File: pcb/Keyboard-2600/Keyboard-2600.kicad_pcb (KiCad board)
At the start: 2 copper layers, 80 x 59.7 mm, 29 parts, among them J1 USB_A, J2 Left Forward Port, J3 Right Forward Port, J4 2600 Joystick Connector, J5 Mini-DIN-6, J6 Expansion Port, SW1 Config Switch-Box, SW2 Reset, U1 ATmega328P-A, U2 74HC4066D_653, U3 74HC4066D_653, Y2 16Mhz

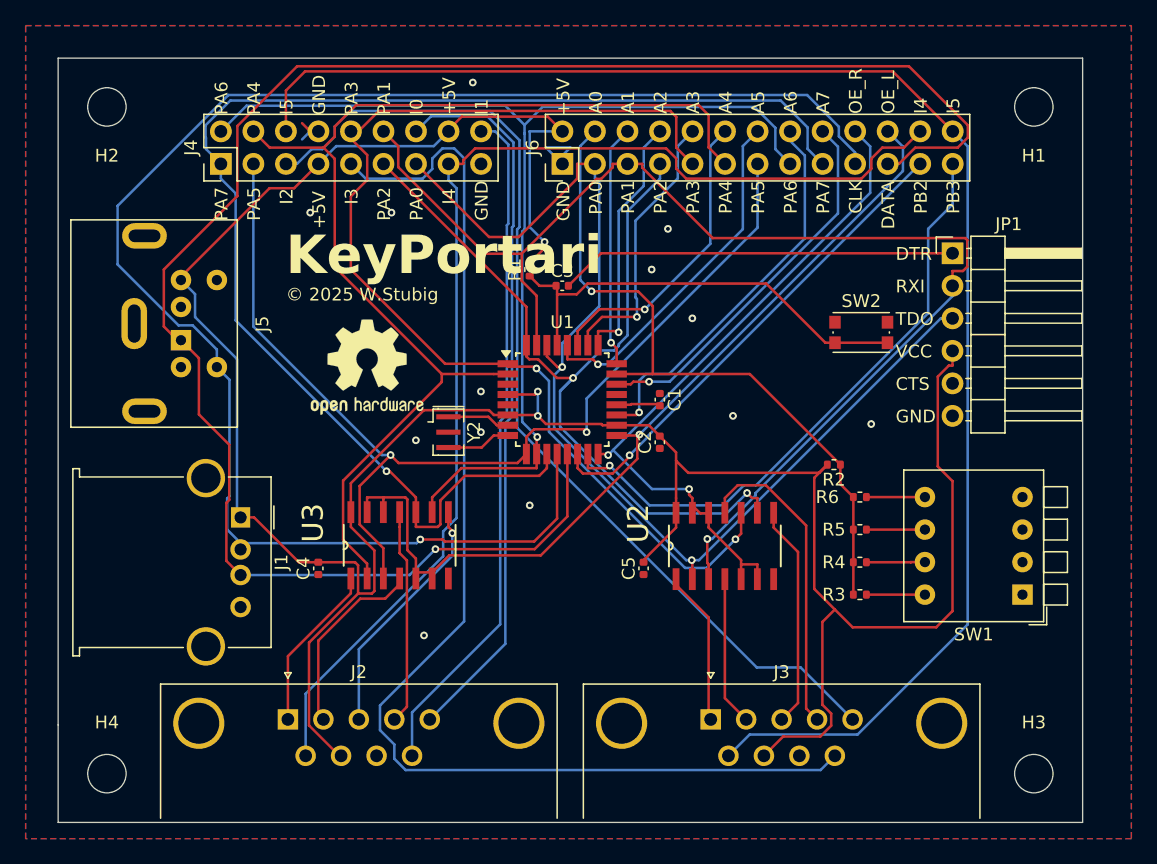
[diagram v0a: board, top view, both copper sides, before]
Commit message: Test board WIP state.
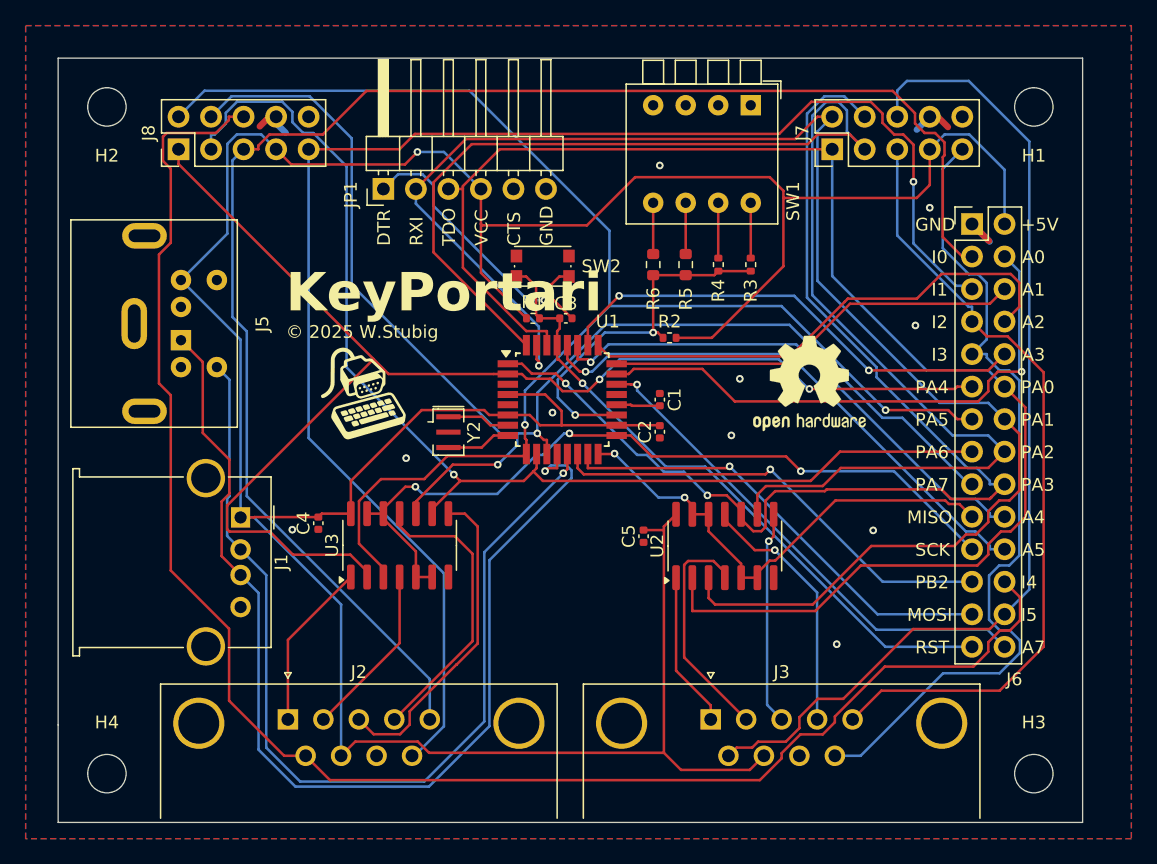
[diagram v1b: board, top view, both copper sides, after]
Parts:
- removed J4: 2600 Joystick Connector, Connector_PinHeader_2.54mm:PinHeader_2x09_P2.54mm_Vertical
- added G***: LOGO, KeyPortari:Logo KeyPortari, F.Cu at (77.5, 90.6)
- added J7: Joystick right, Connector_PinHeader_2.54mm:PinHeader_2x05_P2.54mm_Vertical, F.Cu at (113.8, 70.6)
- added J8: Joystick left, Connector_PinHeader_2.54mm:PinHeader_2x05_P2.54mm_Vertical, F.Cu at (62.7, 70.6)
- J5: footprint 2600-Keyboard:Connector_Mini-DIN_Female_6Pin_2rows -> KeyPortari:Connector_Mini-DIN_Female_6Pin_2rows
- J6: footprint Connector_PinHeader_2.54mm:PinHeader_2x13_P2.54mm_Vertical -> KeyPortari:PinHeader_2x14_P2.54mm_Vertical_KeyPortari_Expansion-Port
- R5, R6: footprint Resistor_SMD:R_0402_1005Metric -> Resistor_SMD:R_0603_1608Metric
- U2, U3: footprint 74HC4066D_653f:SOIC127P600X175-14N -> Package_SO:SOIC-14_3.9x8.7mm_P1.27mm
- moved JP1 44.7 mm to (78.7, 73.7), turned to 90 degrees
- moved SW1 43.7 mm to (107.4, 67.2), turned to -90 degrees
- moved REF** 34.6 mm to (112.0, 88.9)
- moved J6 32.3 mm to (124.7, 76.5), turned to 0 degrees
- moved R3 27.1 mm to (107.4, 79.6), turned to 90 degrees
- moved R4 25.7 mm to (104.9, 79.6), turned to 90 degrees
- moved SW2 25.4 mm to (91.2, 79.8)
- moved R5 24.8 mm to (102.4, 79.6), turned to 90 degrees
- moved R6 24.3 mm to (99.8, 79.6), turned to 90 degrees
- moved R2 16.2 mm to (101.1, 85.3), turned to 0 degrees
- moved R1 3.82 mm to (90.4, 83.8), turned to 180 degrees
- moved C4 3.53 mm to (73.7, 99.8)
- moved C3 2.56 mm to (93.0, 83.8)
- moved C5 2.51 mm to (99.1, 100.8)
- moved C2 0.82 mm to (100.3, 92.7)
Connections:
- C3 pad 1: Net-(U1-~{RESET}/PC6) -> RST
- J6 pad 12: A4 -> PA0
- J6 pad 14: A5 -> PA1
- J6 pad 16: A6 -> PA2
- J6 pad 18: A7 -> PA3
- J6 pad 19: CLK -> OE_R
- J6 pad 20: OE_R -> A4
- J6 pad 21: DATA -> OE_L
- J6 pad 22: OE_L -> A5
- J6 pad 3: PA0 -> I0
- J6 pad 5: PA1 -> I1
- J6 pad 7: PA2 -> I2
- J6 pad 9: PA3 -> I3
- R1 pad 1: Net-(U1-~{RESET}/PC6) -> RST
- R2 pad 1: A0 -> CONF
- R3 pad 1: A0 -> CONF
- R4 pad 1: A0 -> CONF
- R5 pad 1: A0 -> CONF
- R6 pad 1: A0 -> CONF
- SW2 pad 2: Net-(U1-~{RESET}/PC6) -> RST
- U1 pad 12: CLK -> DATA
- U1 pad 13: DATA -> CLK
- U1 pad 19: A6 -> CONF
- U1 pad 29: Net-(U1-~{RESET}/PC6) -> RST
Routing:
- net I0: track 56.7 -> 120.6 mm
- net I1: track 53.4 -> 117.2 mm, vias 0 -> 1
- net DATA: track 141.5 -> 83.3 mm
- net RST: track 0.00 -> 53.9 mm, vias 0 -> 1
- net CLK: track 126.7 -> 75.1 mm
- net PA2: track 70.0 -> 114.8 mm, vias 2 -> 0
- net I5: track 119.8 -> 79.0 mm
- net I4: track 92.3 -> 128.0 mm
- net Net-(U1-~{RESET}/PC6): track 35.1 -> 0.00 mm
- net +5V: track 224.6 -> 257.5 mm, vias 3 -> 1
- net I3: track 96.4 -> 65.6 mm
- net A6: track 30.7 -> 0.00 mm, vias 1 -> 0
- net PA5: track 83.0 -> 112.6 mm
- net CONF: track 0.00 -> 28.7 mm, vias 0 -> 2
- net PA0: track 88.7 -> 117.2 mm, vias 2 -> 0
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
